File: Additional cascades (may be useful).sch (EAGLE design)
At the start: 91 parts, among them J1 S7B-PH-K

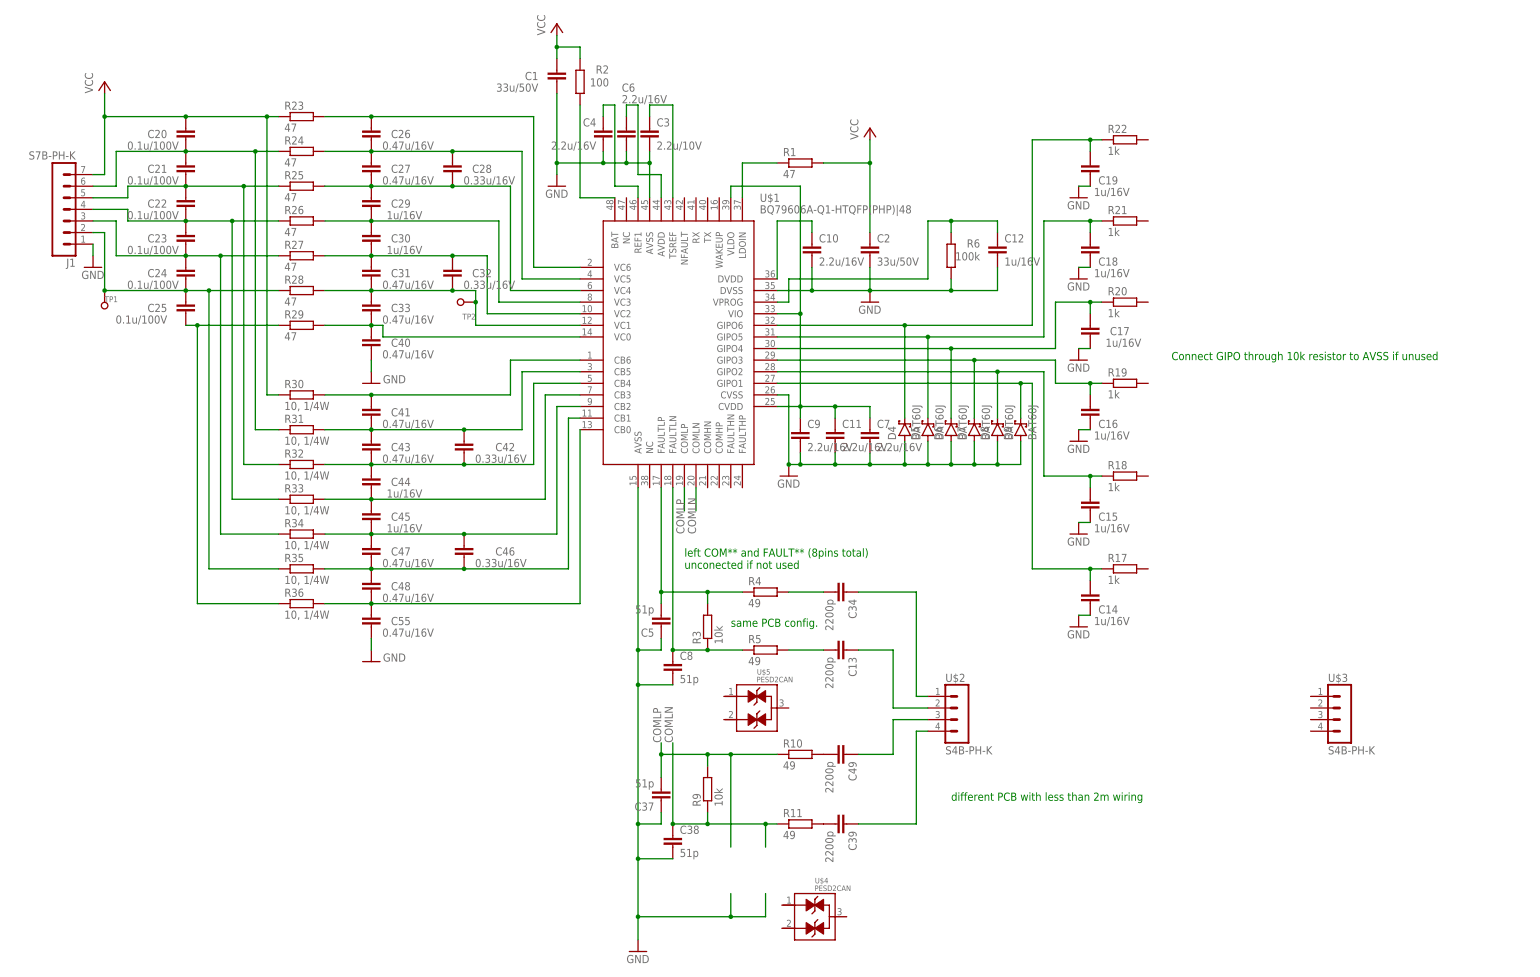
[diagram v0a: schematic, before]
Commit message: some edits
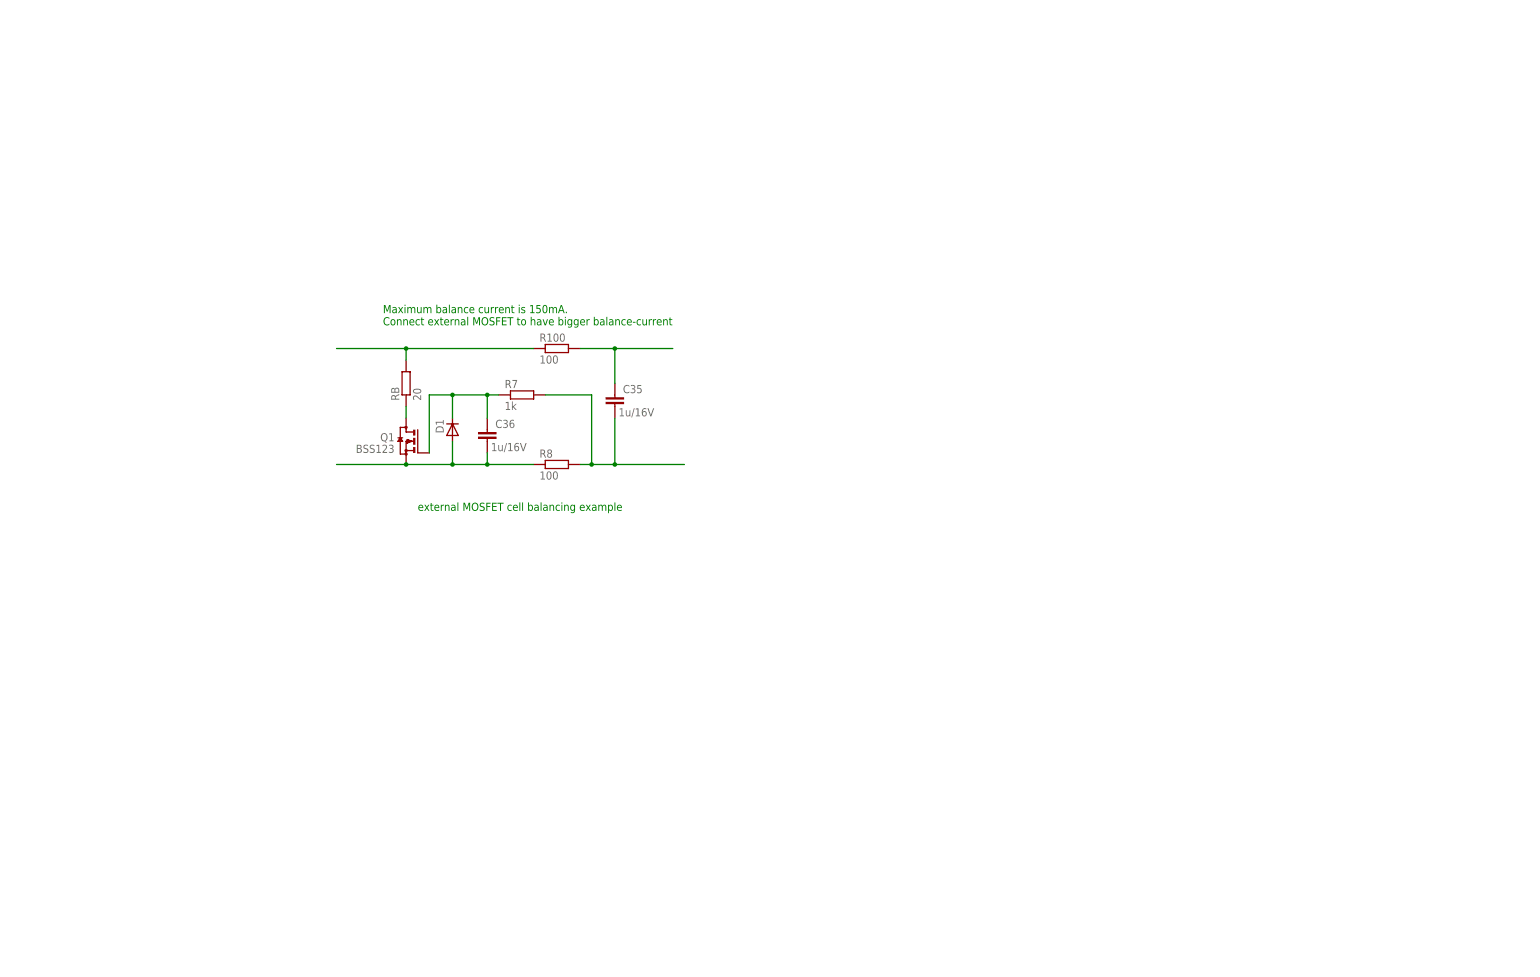
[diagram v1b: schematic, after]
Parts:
- removed C1, C2: 33u/50V, resistor:C-EUC0603
- removed C10, C11, C4, C6, C7, C9: 2.2u/16V, resistor:C-EUC0603
- removed C12, C14, C15, C16, C17, C18, C19, C29, C30, C44, C45: 1u/16V, resistor:C-EUC0603
- removed C13, C34, C39, C49: 2200p, resistor:C-EUC0603
- removed C20, C21, C22, C23, C24, C25: 0.1u/100V, resistor:C-EUC0603
- removed C26, C27, C31, C33, C40, C41, C43, C47, C48, C55: 0.47u/16V, resistor:C-EUC0603
- removed C28, C32, C42, C46: 0.33u/16V, resistor:C-EUC0603
- removed C3: 2.2u/10V, resistor:C-EUC0603
- removed C37, C38, C5, C8: 51p, resistor:C-EUC0603
- removed D4, D5, D6, D7, D8, D9: BAT60J, diode:BAT60J
- removed J1: S7B-PH-K, con-jst-ph:B7B-PH-K
- removed R1, R23, R24, R25, R26, R27, R28, R29: 47, resistor:R-EU_R0603
- removed R10, R11, R4, R5: 49, resistor:R-EU_R0603
- removed R17, R18, R19, R20, R21, R22: 1k, resistor:R-EU_R0603
- removed R2: 100, resistor:R-EU_R0603
- removed R3, R9: 10k, resistor:R-EU_R0603
- removed R30, R31, R32, R33, R34, R35, R36: 10, 1/4W, resistor:R-EU_R0603
- removed R6: 100k, resistor:R-EU_R0603
- removed TP1, TP2: TEST_PAD, testing:TEST_PAD
- removed U$1: BQ79606A-Q1-HTQFP(PHP)|48, texas Instrumets:BQ79606A-Q1-HTQFP(PHP)|48
- removed U$2, U$3: S4B-PH-K, con-jst-ph:S4B-PH-K
- removed U$4, U$5: PESD2CAN, stmicroelectronics:PESD2CAN
- added C35, C36: 1u/16V, resistor:C-EUC0603
- added D1: (no value), eagle-ltspice:DIODE_E-
- added Q1: BSS123, transistor-small-signal:BSS123
- added R100, R8: 100, resistor:R-EU_R0603
- added R7: 1k, resistor:R-EU_R0603
- added RB: 20, resistor:R-EU_R0603
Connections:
- removed net COMLN: C38.1, R11.1, R9.1, U$1.COMLN
- removed net COMLP: C37.2, R10.1, R9.2, U$1.COMLP
- removed net GND: C1.1, C10.2, C11.2, C12.2, C14.1, C15.1, C16.1, C17.1, C18.1, C19.1, C2.2, C3.2, C37.1, C38.2, C4.2, C40.1, C5.1, C55.1, C6.2, C7.2, C8.2, C9.2, D4.A, D5.A, D6.A, D7.A, D8.A, D9.A, J1.1, R6.1, U$1.AVSS@0, U$1.AVSS@1, U$1.CVSS, U$1.DVSS
- removed net N$1: R2.1, U$1.BAT
- removed net N$10: C22.1, C23.2, J1.4, R26.1, R33.1
- removed net N$11: C23.1, C24.2, J1.3, R27.1, R34.1
- removed net N$12: C24.1, C25.2, J1.2, R28.1, R35.1, TP1.P$1
- removed net N$13: C26.1, C27.2, C28.2, R24.2, U$1.VC5
- removed net N$14: C27.1, C28.1, C29.2, R25.2, U$1.VC4
- removed net N$15: C29.1, C30.2, R26.2, U$1.VC3
- removed net N$16: C30.1, C31.2, C32.2, R27.2, U$1.VC2
- removed net N$17: C31.1, C32.1, C33.2, R28.2, TP2.P$1, U$1.VC1
- removed net N$18: C33.1, C40.2, R29.2, U$1.VC0
- removed net N$19: C42.1, C43.1, C44.2, R32.2, U$1.CB4
- removed net N$2: R1.1, U$1.LDOIN
- removed net N$20: C44.1, C45.2, R33.2, U$1.CB3
- removed net N$21: C45.1, C46.2, C47.2, R34.2, U$1.CB2
- removed net N$22: C3.1, U$1.TSREF
- removed net N$23: C48.1, C55.2, R36.2, U$1.CB0
- removed net N$24: C41.1, C42.2, C43.2, R31.2, U$1.CB5
- removed net N$25: C25.1, R29.1, R36.1
- removed net N$26: C26.2, R23.2, U$1.VC6
- removed net N$27: C20.1, C21.2, J1.6, R24.1, R31.1
- removed net N$28: C46.1, C47.1, C48.2, R35.2, U$1.CB1
- removed net N$29: C14.2, D9.C, R17.1, U$1.GIPO1
- removed net N$3: C11.1, C7.1, C9.1, U$1.CVDD, U$1.VIO, U$1.VLDO
- removed net N$30: C19.2, D4.C, R22.1, U$1.GIPO6
- removed net N$31: C18.2, D5.C, R21.1, U$1.GIPO5
- removed net N$32: C17.2, D6.C, R20.1, U$1.GIPO4
- removed net N$33: C16.2, D7.C, R19.1, U$1.GIPO3
- removed net N$34: C15.2, D8.C, R18.1, U$1.GIPO2
- removed net N$35: C5.2, R3.2, R4.1, U$1.FAULTLP
- removed net N$36: C8.1, R3.1, R5.1, U$1.FAULTLN
- removed net N$37: C13.2, R5.2
- removed net N$38: C34.2, R4.2
- removed net N$39: C34.1, U$2.1
- removed net N$4: C6.1, U$1.AVDD
- removed net N$40: C13.1, U$2.2
- removed net N$49: C39.2, R11.2
- removed net N$5: C10.1, U$1.DVDD
- removed net N$50: C49.2, R10.2
- removed net N$51: C49.1, U$2.3
- removed net N$52: C39.1, U$2.4
- removed net N$6: C4.1, U$1.REF1
- removed net N$7: C12.1, R6.2, U$1.VPROG
- removed net N$8: C41.2, R30.2, U$1.CB6
- removed net N$9: C21.1, C22.2, J1.5, R25.1, R32.1
- removed net VCC: C1.2, C2.1, C20.2, J1.7, R1.2, R2.2, R23.1, R30.1
- new net N$41: Q1.D, RB.1
- new net N$42: R100.1, RB.2
- new net N$43: C35.2, R100.2
- new net N$44: C35.1, R7.2, R8.2
- new net N$45: C36.1, D1.C, Q1.S, R8.1
- new net N$46: C36.2, D1.A, Q1.G, R7.1
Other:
- note added: "Maximum balance current is 150mA. Connect external MOSFET to have bigger balance-current"
- note added: "external MOSFET cell balancing example"
- note removed: "Connect GIPO through 10k resistor to AVSS if unused"
- note removed: "different PCB with less than 2m wiring"
- note removed: "left COM** and FAULT** (8pins total) unconected if not used"
- note removed: "same PCB config."
